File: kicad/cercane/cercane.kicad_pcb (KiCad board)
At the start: 2 copper layers, 2 parts, among them U1 ATtiny45-20SU, U2 NRF24L01_Breakout

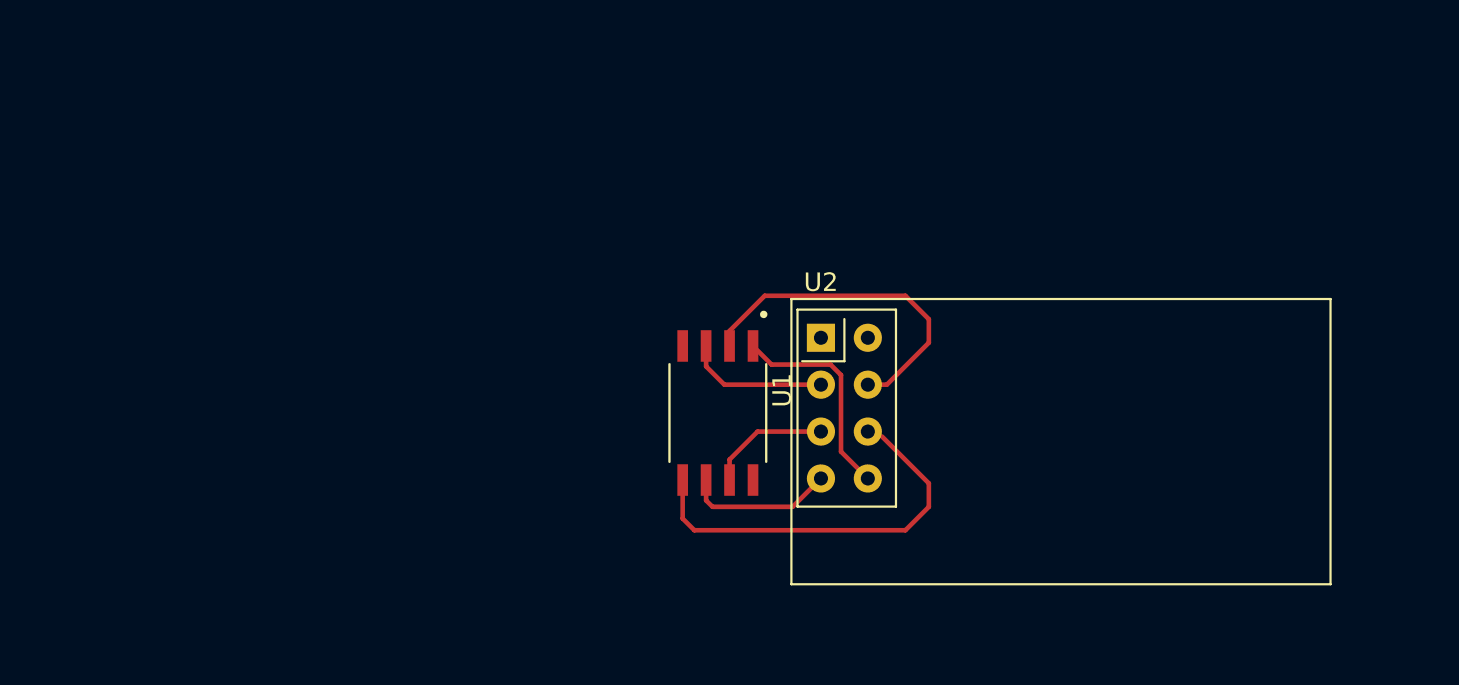
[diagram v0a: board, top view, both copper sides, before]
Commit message: new PCB
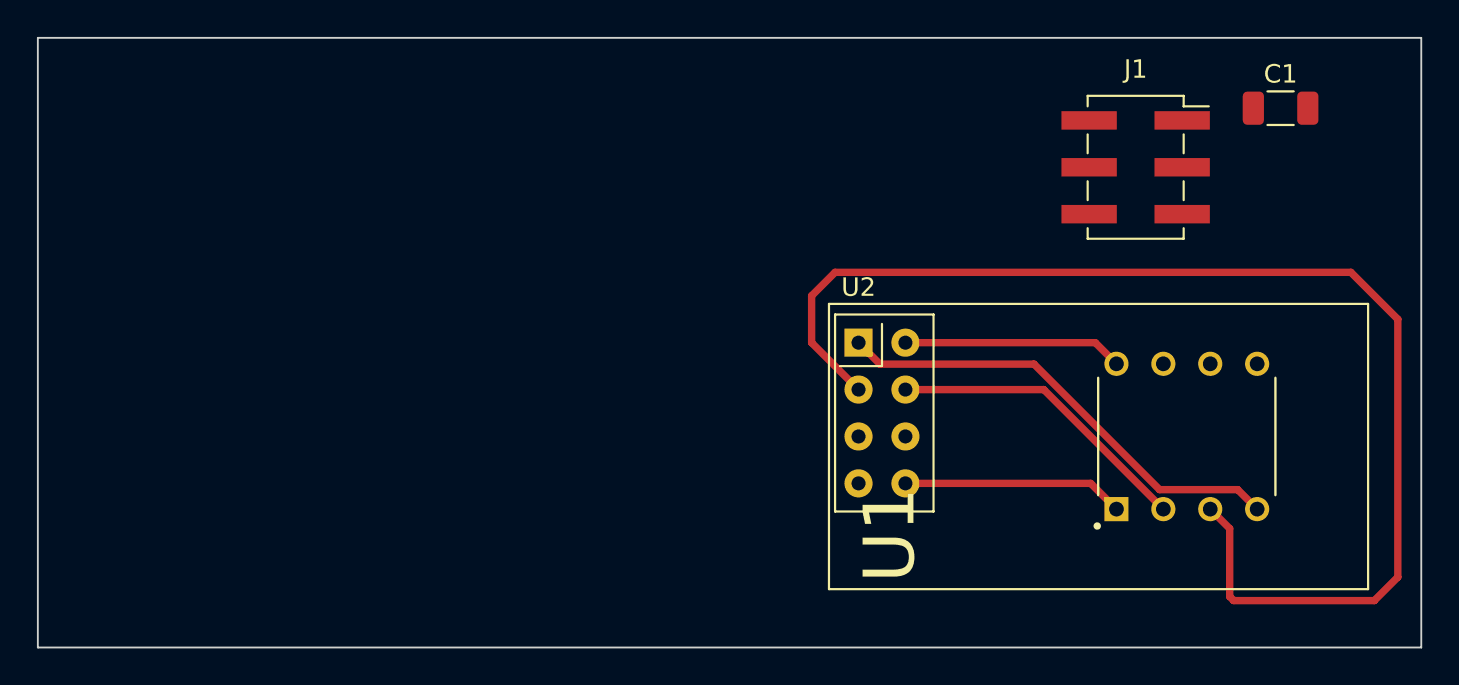
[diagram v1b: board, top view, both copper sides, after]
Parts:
- added C1: 100nF, Capacitor_SMD:C_1206_3216Metric, F.Cu at (179.1, 58.4)
- added J1: Conn_02x03_Odd_Even, Connector_PinSocket_2.54mm:PinSocket_2x03_P2.54mm_Vertical_SMD, F.Cu at (171.2, 61.6)
- U1: value ATtiny45-20SU -> ATtiny45-20PU; footprint ATTINY85-20SU:SOIC127P798X216-8N -> ATTINY45-20PU:DIP787W46P254L927H533Q8
- moved U1 25.4 mm to (174.0, 76.2), turned to 90 degrees
- moved U2 2.05 mm to (156.2, 71.1)
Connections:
- net Net-(U1-Pad6) renamed /MISO
- net VCC renamed +3V3
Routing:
- net Net-(U1-Pad3): track 7.74 -> 68.3 mm
- net GND: track 0.00 -> 25.3 mm
- net Net-(U1-Pad5): track 21.1 -> 0.00 mm
- net +3V3: track 0.00 -> 11.9 mm
- net /MISO: track 8.10 -> 0.00 mm
- net Net-(U1-Pad7): track 6.68 -> 0.00 mm
- net Net-(U1-Pad2): track 18.4 -> 16.7 mm
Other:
- board outline added: 74.9 x 33 mm
- net class Default: trace_width 0.25 -> 0.4
- rule trace_min: 0.2 -> 0.3
